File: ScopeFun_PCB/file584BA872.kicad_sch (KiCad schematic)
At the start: 54 parts, among them U14 SN74AUP1T17DCKR, U29 CYUSB3014, U30 M24M02-DR, X1 X_Crystal_19.2Mhz

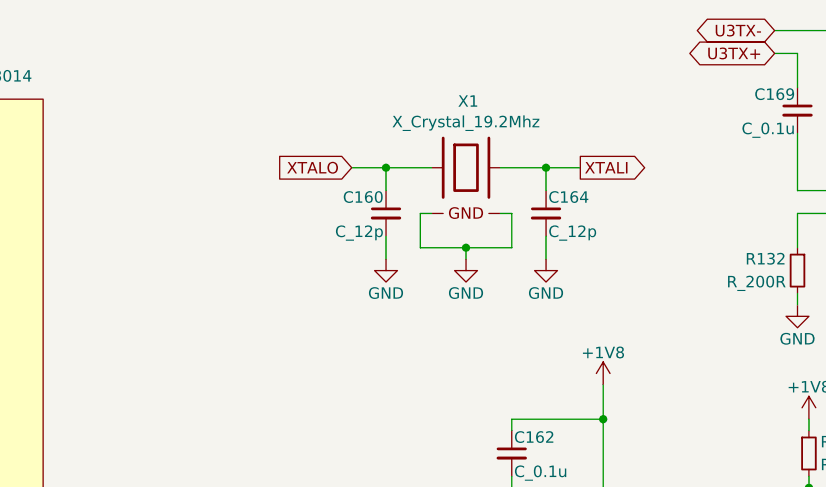
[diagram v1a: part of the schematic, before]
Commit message: 260420
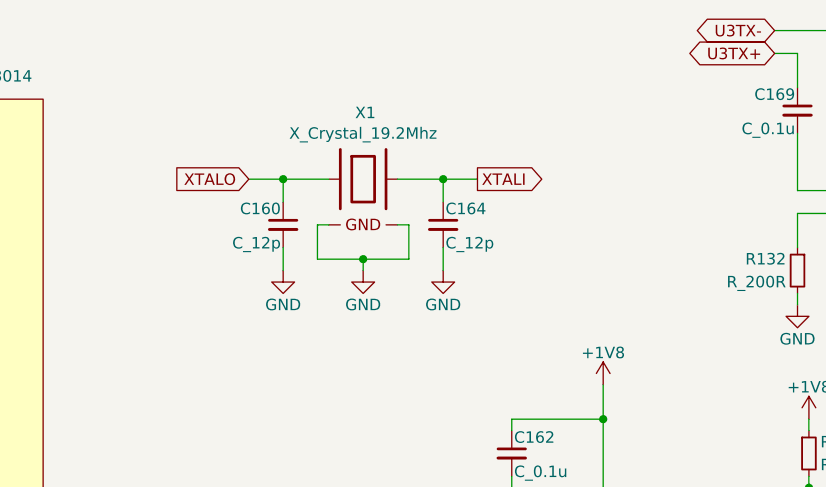
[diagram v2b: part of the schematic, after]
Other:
- moved on the sheet: C160, C164, X1
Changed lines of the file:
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@@
 	)
 	(junction
-		(at 177.8 34.29)
+		(at 166.37 35.56)
 		(diameter 0)
 		(color 0 0 0 0)
@@
 	)
 	(junction
-		(at 195.58 34.29)
+		(at 184.15 35.56)
 		(diameter 0)
 		(color 0 0 0 0)
@@
 	)
 	(junction
-		(at 186.69 43.18)
+		(at 175.26 44.45)
 		(diameter 0)
 		(color 0 0 0 0)
@@
 	(wire
 		(pts
-			(xy 177.8 44.45) (xy 177.8 41.91)
+			(xy 166.37 45.72) (xy 166.37 43.18)
 		)
 		(stroke
@@
 	(wire
 		(pts
-			(xy 191.77 39.37) (xy 190.5 39.37)
+			(xy 180.34 40.64) (xy 179.07 40.64)
 		)
 		(stroke
@@
 	(wire
 		(pts
-			(xy 186.69 43.18) (xy 191.77 43.18)
+			(xy 175.26 44.45) (xy 180.34 44.45)
 		)
 		(stroke
@@
 	(wire
 		(pts
-			(xy 191.77 43.18) (xy 191.77 39.37)
+			(xy 180.34 44.45) (xy 180.34 40.64)
 		)
 		(stroke
@@
 	(wire
 		(pts
-			(xy 173.99 34.29) (xy 177.8 34.29)
+			(xy 162.56 35.56) (xy 166.37 35.56)
 		)
 		(stroke
@@
 	(wire
 		(pts
-			(xy 195.58 34.29) (xy 199.39 34.29)
+			(xy 184.15 35.56) (xy 187.96 35.56)
 		)
 		(stroke
@@
 	(wire
 		(pts
-			(xy 190.5 34.29) (xy 195.58 34.29)
+			(xy 179.07 35.56) (xy 184.15 35.56)
 		)
 		(stroke
@@
 	(wire
 		(pts
-			(xy 182.88 39.37) (xy 181.61 39.37)
+			(xy 171.45 40.64) (xy 170.18 40.64)
 		)
 		(stroke
@@
 	(wire
 		(pts
-			(xy 195.58 44.45) (xy 195.58 41.91)
+			(xy 184.15 45.72) (xy 184.15 43.18)
 		)
 		(stroke
@@
 	(wire
 		(pts
-			(xy 181.61 39.37) (xy 181.61 43.18)
+			(xy 170.18 40.64) (xy 170.18 44.45)
 		)
 		(stroke
@@
 	(wire
 		(pts
-			(xy 181.61 43.18) (xy 186.69 43.18)
+			(xy 170.18 44.45) (xy 175.26 44.45)
 		)
 		(stroke
@@
 	(wire
 		(pts
-			(xy 195.58 34.29) (xy 195.58 36.83)
+			(xy 184.15 35.56) (xy 184.15 38.1)
 		)
 		(stroke
@@
 	(wire
 		(pts
-			(xy 177.8 34.29) (xy 177.8 36.83)
+			(xy 166.37 35.56) (xy 166.37 38.1)
 		)
 		(stroke
@@
 	(wire
 		(pts
-			(xy 177.8 34.29) (xy 182.88 34.29)
+			(xy 166.37 35.56) (xy 171.45 35.56)
 		)
 		(stroke
@@
 	(wire
 		(pts
-			(xy 186.69 44.45) (xy 186.69 43.18)
+			(xy 175.26 45.72) (xy 175.26 44.45)
 		)
 		(stroke
@@
 	(global_label "XTALI"
 		(shape output)
-		(at 199.39 34.29 0)
+		(at 187.96 35.56 0)
 		(effects
 			(font
@@
 		)
 		(property "Intersheetrefs" "${INTERSHEET_REFS}"
-			(at 199.39 34.29 0)
+			(at 187.96 35.56 0)
 			(hide yes)
 			(show_name no)
@@
 	(global_label "XTALO"
 		(shape input)
-		(at 173.99 34.29 180)
+		(at 162.56 35.56 180)
 		(effects
 			(font
@@
 		)
 		(property "Intersheetrefs" "${INTERSHEET_REFS}"
-			(at 173.99 34.29 0)
+			(at 162.56 35.56 0)
 			(hide yes)
 			(show_name no)
@@
 		(lib_name "GND_47")
 		(lib_id "Scopefun_v2-rescue:GND")
-		(at 177.8 44.45 0)
+		(at 166.37 45.72 0)
 		(unit 1)
 		(body_style 1)
@@
 		(dnp no)
 		(property "Reference" "#PWR0275"
-			(at 177.8 50.8 0)
+			(at 166.37 52.07 0)
 			(hide yes)
 			(show_name no)
@@
 		)
 		(property "Value" "GND"
-			(at 177.8 48.26 0)
+			(at 166.37 49.53 0)
 			(show_name no)
 			(do_not_autoplace no)
@@
 		)
 		(property "Footprint" ""
-			(at 177.8 44.45 0)
+			(at 166.37 45.72 0)
 			(show_name no)
 			(do_not_autoplace no)
@@
 		)
 		(property "Datasheet" ""
-			(at 177.8 44.45 0)
+			(at 166.37 45.72 0)
 			(show_name no)
 			(do_not_autoplace no)
@@
 		)
 		(property "Description" ""
-			(at 177.8 44.45 0)
+			(at 166.37 45.72 0)
 			(show_name no)
 			(do_not_autoplace no)
@@
 		(lib_name "GND_45")
 		(lib_id "Scopefun_v2-rescue:GND")
-		(at 195.58 44.45 0)
+		(at 184.15 45.72 0)
 		(unit 1)
 		(body_style 1)
@@
 		(dnp no)
 		(property "Reference" "#PWR0276"
-			(at 195.58 50.8 0)
+			(at 184.15 52.07 0)
 			(hide yes)
 			(show_name no)
@@
 		)
 		(property "Value" "GND"
-			(at 195.58 48.26 0)
+			(at 184.15 49.53 0)
 			(show_name no)
 			(do_not_autoplace no)
@@
 		)
 		(property "Footprint" ""
-			(at 195.58 44.45 0)
+			(at 184.15 45.72 0)
 			(show_name no)
 			(do_not_autoplace no)
@@
 		)
 		(property "Datasheet" ""
-			(at 195.58 44.45 0)
+			(at 184.15 45.72 0)
 			(show_name no)
 			(do_not_autoplace no)
@@
 		)
 		(property "Description" ""
-			(at 195.58 44.45 0)
+			(at 184.15 45.72 0)
 			(show_name no)
 			(do_not_autoplace no)
@@
 		(lib_name "GND_46")
 		(lib_id "Scopefun_v2-rescue:GND")
-		(at 186.69 44.45 0)
+		(at 175.26 45.72 0)
 		(unit 1)
 		(body_style 1)
@@
 		(dnp no)
 		(property "Reference" "#PWR0277"
-			(at 186.69 50.8 0)
+			(at 175.26 52.07 0)
 			(hide yes)
 			(show_name no)
@@
 		)
 		(property "Value" "GND"
-			(at 186.69 48.26 0)
+			(at 175.26 49.53 0)
 			(show_name no)
 			(do_not_autoplace no)
@@
 		)
 		(property "Footprint" ""
-			(at 186.69 44.45 0)
+			(at 175.26 45.72 0)
 			(show_name no)
 			(do_not_autoplace no)
@@
 		)
 		(property "Datasheet" ""
-			(at 186.69 44.45 0)
+			(at 175.26 45.72 0)
 			(show_name no)
 			(do_not_autoplace no)
@@
 		)
 		(property "Description" ""
-			(at 186.69 44.45 0)
+			(at 175.26 45.72 0)
 			(show_name no)
 			(do_not_autoplace no)
@@
 	(symbol
 		(lib_id "ScopefunParts:X_Crystal_19.2Mhz")
-		(at 186.69 34.29 0)
+		(at 175.26 35.56 0)
 		(unit 1)
 		(body_style 1)
@@
 		(dnp no)
 		(property "Reference" "X1"
-			(at 186.944 26.924 0)
+			(at 175.514 28.194 0)
 			(show_name no)
 			(do_not_autoplace no)
@@
 		)
 		(property "Value" "X_Crystal_19.2Mhz"
-			(at 186.69 29.21 0)
+			(at 175.26 30.48 0)
 			(show_name no)
 			(do_not_autoplace no)
@@
 		)
 		(property "Footprint" "ScopefunPackagesLibrary:XTAL-4"
-			(at 186.69 44.958 0)
+			(at 175.26 46.228 0)
 			(hide yes)
 			(show_name no)
@@
 		)
 		(property "Datasheet" "https://www.pericom.com/assets/Datasheets/FL1920031.pdf"
-			(at 186.944 42.418 0)
+			(at 175.514 43.688 0)
 			(hide yes)
 			(show_name no)
@@
 		)
 		(property "Description" "Quartz crystal 19.2 Mhz 10ppm"
-			(at 186.69 21.59 0)
+			(at 175.26 22.86 0)
 			(hide yes)
 			(show_name no)
@@
 		)
 		(property "MFG Part#" "FL1920031"
-			(at 186.69 24.13 0)
+			(at 175.26 25.4 0)
 			(hide yes)
 			(show_name no)
@@
 	(symbol
 		(lib_id "ScopefunParts:C_12p")
-		(at 177.8 39.37 0)
+		(at 166.37 40.64 0)
 		(mirror y)
 		(unit 1)
@@
 		(dnp no)
 		(property "Reference" "C160"
-			(at 177.546 37.592 0)
+			(at 166.116 38.862 0)
 			(show_name no)
 			(do_not_autoplace no)
@@
 		)
 		(property "Value" "C_12p"
-			(at 177.546 41.402 0)
+			(at 166.116 42.672 0)
 			(show_name no)
 			(do_not_autoplace no)
@@
 		)
 		(property "Footprint" "ScopefunPackagesLibrary:C_0603"
-			(at 177.8 44.45 0)
+			(at 166.37 45.72 0)
 			(hide yes)
 			(show_name no)
@@
 		)
 		(property "Datasheet" ""
-			(at 177.546 37.592 0)
+			(at 166.116 38.862 0)
 			(hide yes)
 			(show_name no)
@@
 		)
 		(property "Description" "MLCC - SMD/SMT 0603 50V C0G 5%"
-			(at 176.53 33.02 0)
+			(at 165.1 34.29 0)
 			(hide yes)
 			(show_name no)
@@
 		)
 		(property "MFG Part#" "CGA3E2C0G1H120J080AA"
-			(at 175.006 35.052 0)
+			(at 163.576 36.322 0)
 			(hide yes)
 			(show_name no)
@@
 	(symbol
 		(lib_id "ScopefunParts:C_12p")
-		(at 195.58 39.37 0)
+		(at 184.15 40.64 0)
 		(unit 1)
 		(body_style 1)
@@
 		(dnp no)
 		(property "Reference" "C164"
-			(at 195.834 37.592 0)
+			(at 184.404 38.862 0)
 			(show_name no)
 			(do_not_autoplace no)
@@
 		)
 		(property "Value" "C_12p"
-			(at 195.834 41.402 0)
+			(at 184.404 42.672 0)
 			(show_name no)
 			(do_not_autoplace no)
@@
 		)
 		(property "Footprint" "ScopefunPackagesLibrary:C_0603"
-			(at 195.58 44.45 0)
+			(at 184.15 45.72 0)
 			(hide yes)
 			(show_name no)
@@
 		)
 		(property "Datasheet" ""
-			(at 195.834 37.592 0)
+			(at 184.404 38.862 0)
 			(hide yes)
 			(show_name no)
@@
 		)
 		(property "Description" "MLCC - SMD/SMT 0603 50V C0G 5%"
-			(at 196.85 33.02 0)
+			(at 185.42 34.29 0)
 			(hide yes)
 			(show_name no)
@@
 		)
 		(property "MFG Part#" "CGA3E2C0G1H120J080AA"
-			(at 198.374 35.052 0)
+			(at 186.944 36.322 0)
 			(hide yes)
 			(show_name no)
